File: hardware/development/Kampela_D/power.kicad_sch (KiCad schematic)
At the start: 83 parts

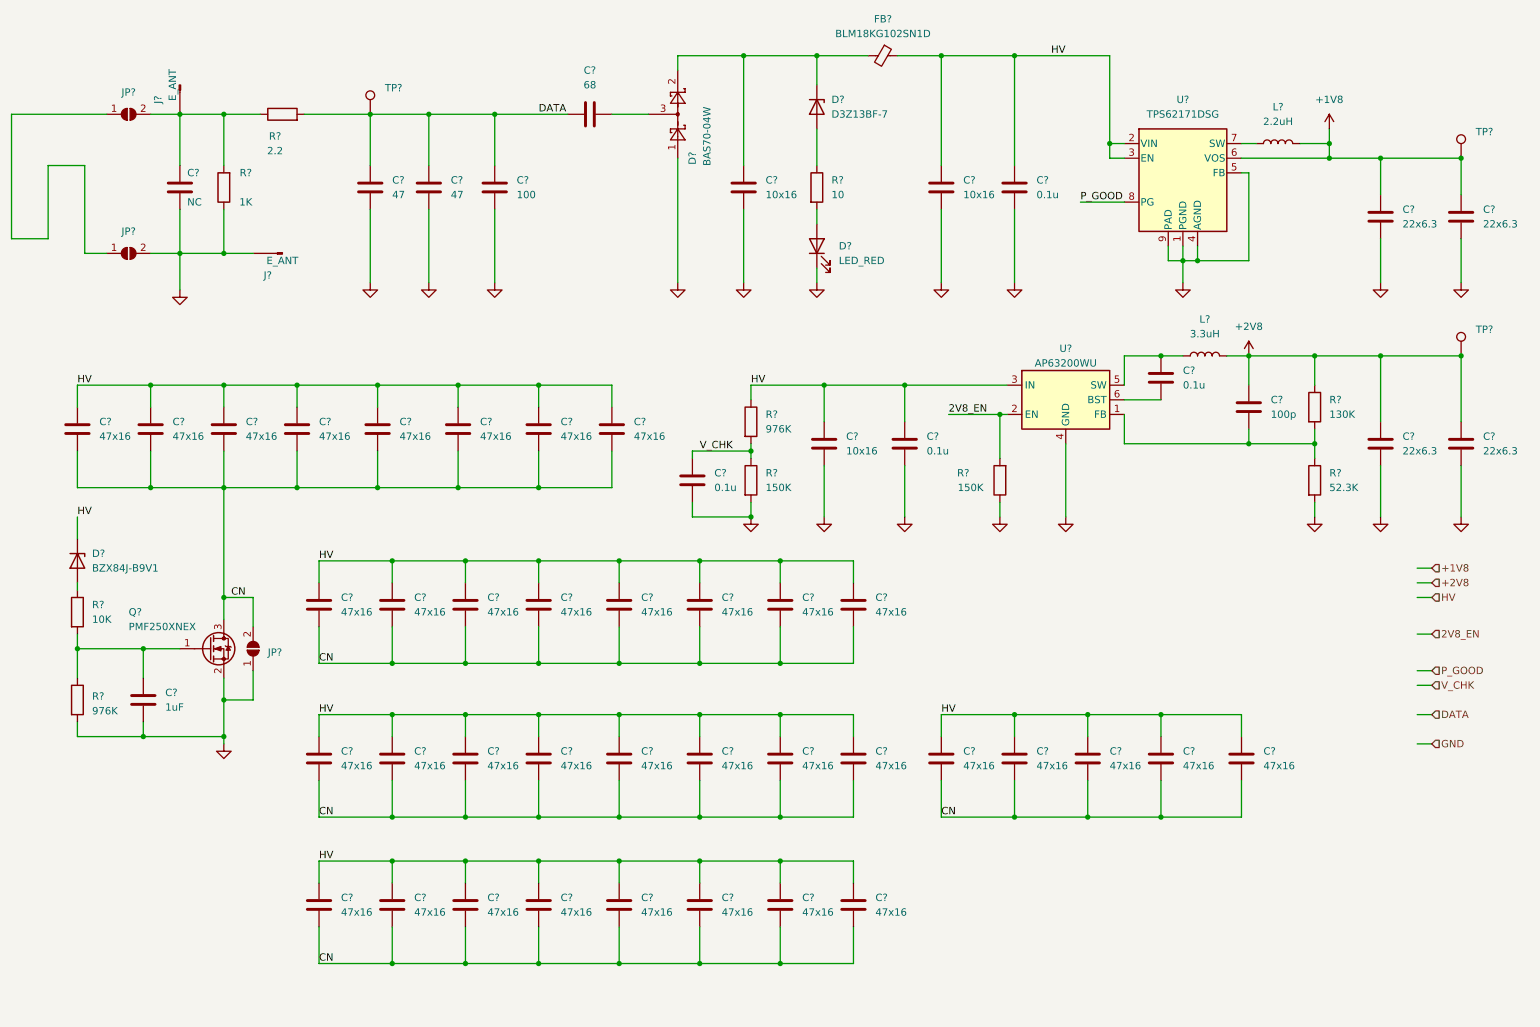
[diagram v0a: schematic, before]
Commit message: major: first device prototype (#24)
* feat: initial routing

* feat: pcb labels

* feat: update C1 version; add D version and tag
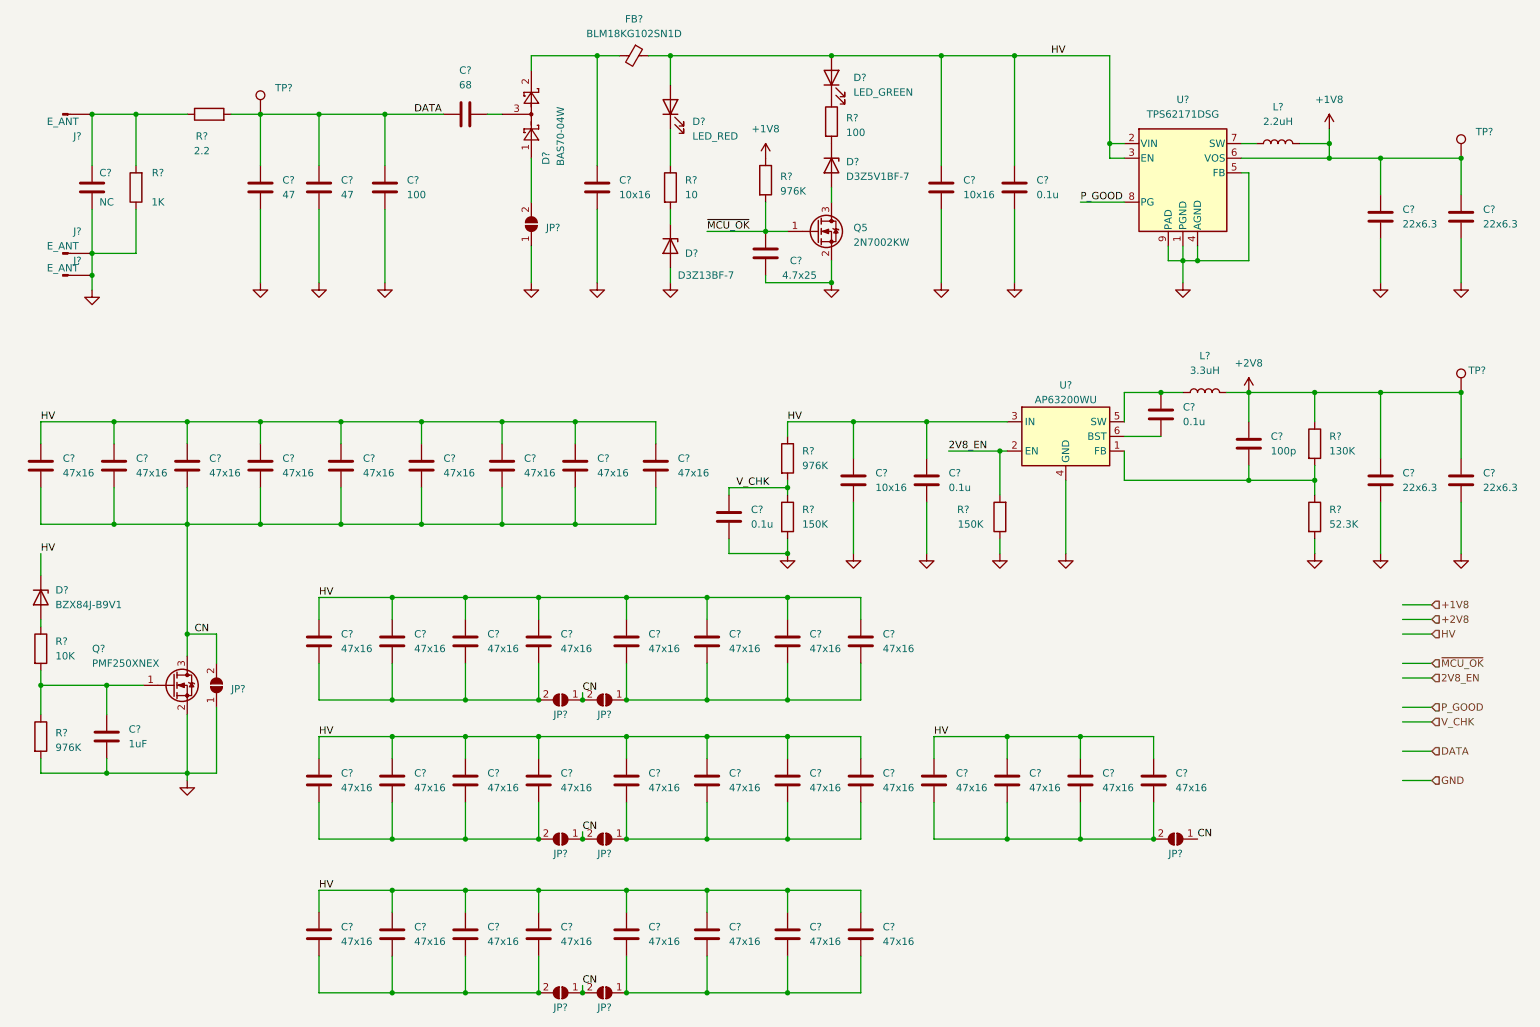
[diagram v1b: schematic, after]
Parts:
- removed C? (x29): 47x16, Capacitor_SMD:C_1210_3225Metric, symbol Device:C
- removed D?: D3Z13BF-7, Diode_SMD:D_SOD-323F, symbol Device:D_Zener
- removed D?: LED_RED, LED_SMD:LED_0603_1608Metric, symbol Device:LED
- removed FB?: BLM18KG102SN1D, Inductor_SMD:L_0603_1608Metric, symbol Device:FerriteBead_Small
- removed JP? (x2): SolderJumper_2_Open, Jumper:SolderJumper-2_P1.3mm_Open_RoundedPad1.0x1.5mm, symbol Jumper:SolderJumper_2_Open
- added C? (x29): 47x16, Capacitor_SMD:C_1210_3225Metric, symbol Device:C
- added C?: 4.7x25, Capacitor_SMD:C_0402_1005Metric, symbol Device:C
- added D?: D3Z5V1BF-7, Diode_SMD:D_SOD-323F, symbol Device:D_Zener
- added D?: LED_GREEN, LED_SMD:LED_0603_1608Metric, symbol Device:LED
- added D?: LED_RED, LED_SMD:LED_0603_1608Metric, symbol Device:LED
- added D?: D3Z13BF-7, Diode_SMD:D_SOD-323F, symbol Device:D_Zener
- added FB?: BLM18KG102SN1D, Inductor_SMD:L_0603_1608Metric, symbol Device:FerriteBead_Small
- added J?: E_ANT, MyLib:TestPoint_Pad_2.4x3.5mm, symbol Connector:Conn_01x01_Male
- added JP? (x8): SolderJumper_2_Open, MyLib:SolderJumper_0.8.x1mm, symbol Jumper:SolderJumper_2_Open
- added Q5: 2N7002KW, Package_TO_SOT_SMD:SOT-323_SC-70, symbol Transistor_FET:2N7002
- added R?: 976K, Resistor_SMD:R_0402_1005Metric, symbol Device:R
- added R?: 100, Resistor_SMD:R_0402_1005Metric, symbol Device:R
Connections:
- net +1V8: now also R?.1
- net CN: now also C?.1, JP?.1 (A), JP?.1 (A), JP?.1 (A), JP?.1 (A), JP?.2 (B), JP?.2 (B), JP?.2 (B)
- net GND: now also C?.1, D?.2 (A), J?.1 (Pin_1), JP?.1 (A), Q5.2 (S); no longer D?.1
- net HV: now also C?.2, C?.2, C?.2, C?.2, C?.2, C?.2, C?.2, C?.2, C?.2, C?.2, C?.2, C?.2, C?.2, C?.2, C?.2, C?.2, C?.2, C?.2, C?.2, C?.2, C?.2, C?.2, C?.2, C?.2, C?.2, C?.2, C?.2, C?.2, C?.2, D?.2 (A), D?.2 (A), FB?.1
- net at R?.1: now also D?.1 (K)
- net at R?.2: now also D?.1 (K)
- net at C?.2, D?.2: now also FB?.2
- new net: C?.1, C?.1, C?.1, C?.1, JP?.2 (B) (x4)
- new net: C?.1, C?.1, C?.1, C?.1, JP?.1 (A) (x3)
- new net: D?.1 (K), R?.2
- new net: D?.2 (A), Q5.3 (D)
- new net: D?.1, JP?.2 (B)
- new net: D?.1 (K), R?.1
- new net ~{MCU_OK}: C?.2, Q5.1 (G), R?.2
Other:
- moved on the sheet: C?, D?, J?, JP?, L?, Q?, R?, TP?, U?
